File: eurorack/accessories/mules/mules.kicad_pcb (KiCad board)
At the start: 2 copper layers, 23.4 x 14.7 mm, 6 parts, among them J1 AudioPlug2, J2 AudioPlug2, J3 AudioJack3

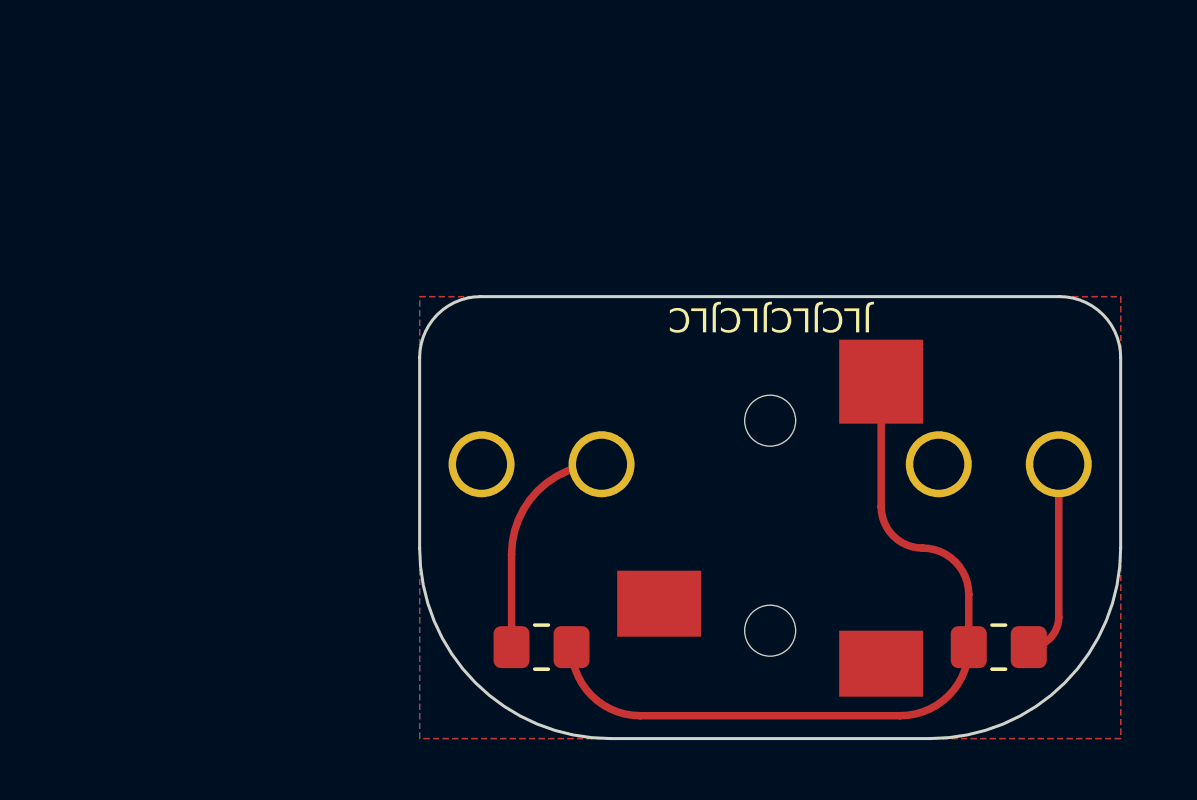
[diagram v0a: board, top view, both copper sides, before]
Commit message: final mules v1 design
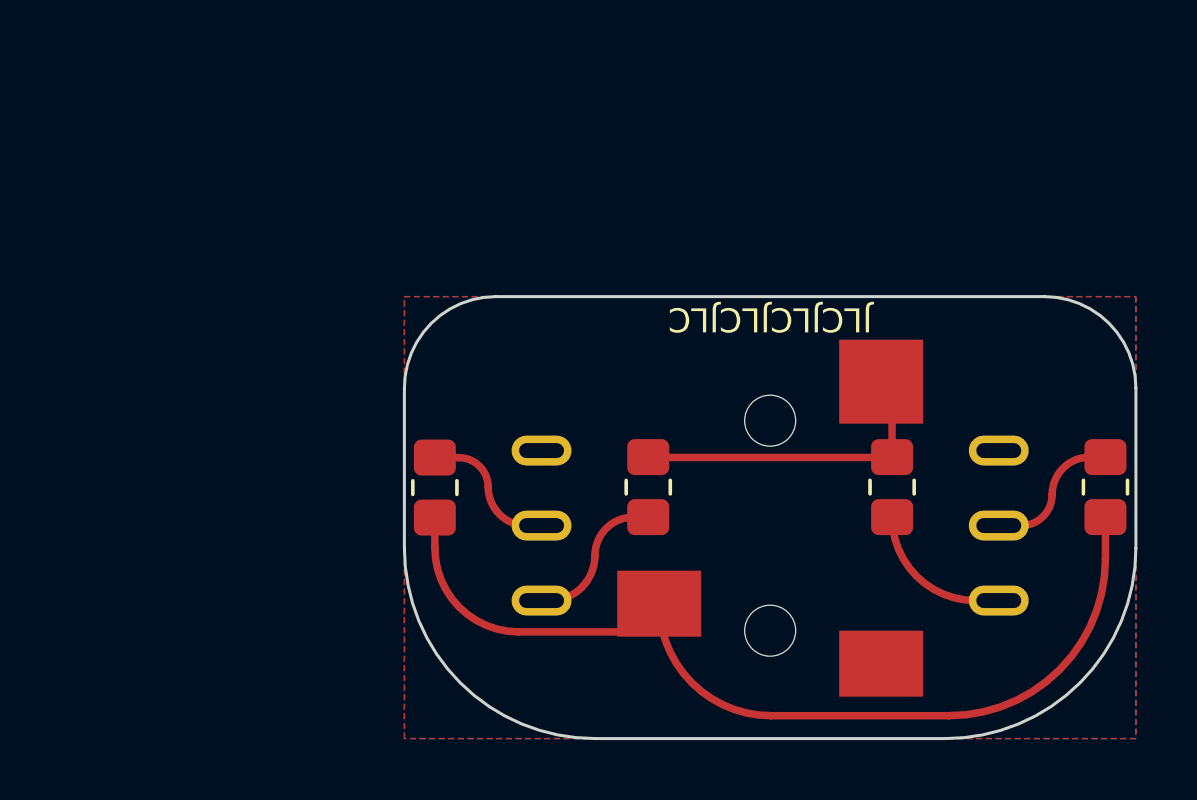
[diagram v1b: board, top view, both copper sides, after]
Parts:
- added R3: 1k, Resistor_SMD:R_0805_2012Metric_Pad1.20x1.40mm_HandSolder, F.Cu at (151.4, 104.9)
- added R4: 1k, Resistor_SMD:R_0805_2012Metric_Pad1.20x1.40mm_HandSolder, F.Cu at (173.7, 104.9)
- J1, J2: value AudioPlug2 -> AudioPlug3; footprint Pale Slim Ghost:Kobiconn 173-35MPTIP-EX 3.5mm Audio Plug -> Pale Slim Ghost:Plug_3.5mm_CUI_SP-3533
- moved R1 6.41 mm to (158.5, 104.9), turned to 90 degrees
- moved R2 6.41 mm to (166.6, 104.9), turned to 90 degrees
- moved J1 2.04 mm to (154.9, 106.2)
- moved J2 2.04 mm to (170.2, 106.2)
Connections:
- J3 pad R: GND -> Net-(J3-PadR)
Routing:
- net Net-(J3-PadR): track 0.00 -> 31.5 mm
- net Net-(R1-Pad2): track 26.1 -> 10.8 mm
- net Net-(J2-PadR): track 0.00 -> 4.77 mm
- net Net-(J1-PadR): track 0.00 -> 4.76 mm
- net Net-(R1-Pad1): track 7.69 -> 5.03 mm
- net Net-(R2-Pad1): track 6.63 -> 5.03 mm
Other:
- board size 23.4 x 14.7 mm -> 24.4 x 14.7 mm

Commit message: assorted changes ig from opening things in kicad 7
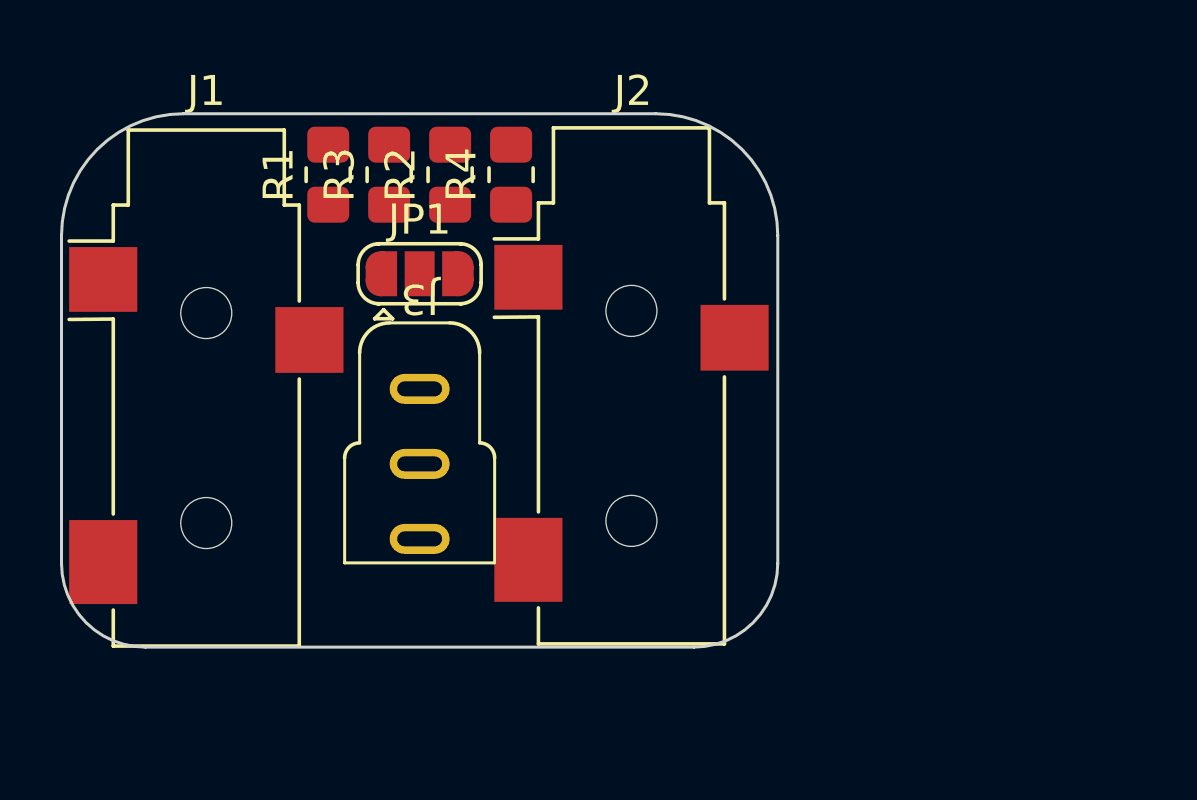
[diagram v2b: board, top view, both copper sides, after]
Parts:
- added JP1: SolderJumper_3_Open, Jumper:SolderJumper-3_P1.3mm_Open_RoundedPad1.0x1.5mm, F.Cu at (150.9, 97.8)
- J1, J2: value AudioPlug3 -> AudioJack3; footprint Pale Slim Ghost:Plug_3.5mm_CUI_SP-3533 -> Connector_Audio:Jack_3.5mm_CUI_SJ-3523-SMT_Horizontal
- J3: value AudioJack3 -> AudioPlug3; footprint Connector_Audio:Jack_3.5mm_CUI_SJ-3523-SMT_Horizontal -> Pale Slim Ghost:Plug_3.5mm_CUI_SP-3533
- moved R4 22.4 mm to (153.9, 94.5), turned to 90 degrees
- moved R2 18.0 mm to (151.9, 94.5)
- moved R1 14.9 mm to (147.8, 94.5)
- moved J2 13.0 mm to (158.0, 101.6)
- moved G*** 12.7 mm to (151.1, 101.1)
- moved J1 12.1 mm to (143.8, 101.6)
- moved J3 12.1 mm to (150.9, 104.1)
- moved R3 10.5 mm to (149.9, 94.5), turned to 90 degrees
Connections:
- J3 pad T: Net-(R1-Pad2) -> Net-(J3-PadT)
- R2 pad 2: Net-(R1-Pad2) -> Net-(J3-PadT)
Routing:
- net Net-(J3-PadR): track 31.5 -> 0.00 mm
- net Net-(R1-Pad2): track 10.8 -> 0.00 mm
- net Net-(J1-PadT): track 5.03 -> 0.00 mm
- net Net-(J2-PadT): track 5.03 -> 0.00 mm
- net Net-(J2-PadR): track 4.77 -> 0.00 mm
- net Net-(J1-PadR): track 4.76 -> 0.00 mm
- removed copper zone on B.Cu, net GND
- removed copper zone on F.Cu, net GND
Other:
- board size 24.4 x 14.7 mm -> 23.9 x 17.8 mm
- board text removed: "JLCJLCJLCJLC"
